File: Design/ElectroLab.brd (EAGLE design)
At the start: 175 x 100 mm, 229 parts, among them IC11 PAM8403, IC13 74HC08DD, IC14 74HC04DD, IC15 74HC32S14-13, IC3 LM324DTD, IC4 LM324DTD, IC6 MC74HC112ADR2G, IC7 MC74HC112ADR2G, IC8 TLC555CDR, IC9 TP4056, P1 SLIDE_POT_20MM, T1 MMBT2222A, T2 T_NPNMMBT2222A-1P_CHANGJ_SOT2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, T3 T_NPNMMBT2222A-1P_CHANGJ_SOT2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, T4 T_PNPMMBT5401_CHANGJ_SOT23-BEC, T5 T_PNPMMBT5401_CHANGJ_SOT23-BEC, U1 ADXL335, U2 GAS_SENSOR, U3 AMS1117-3.3VSMD, X8 USB-C-POWER

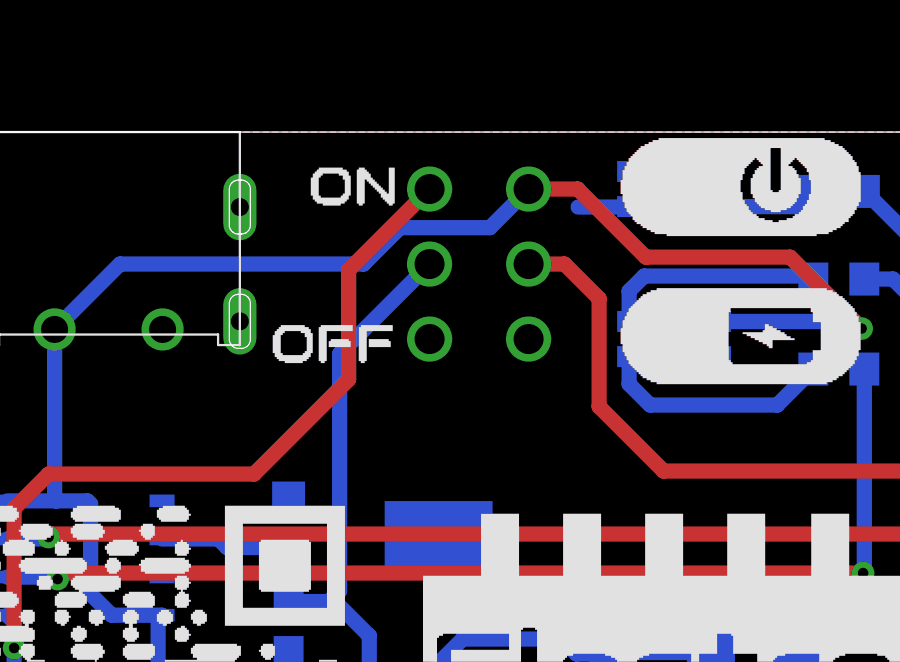
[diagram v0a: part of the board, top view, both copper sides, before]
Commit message: Added design files
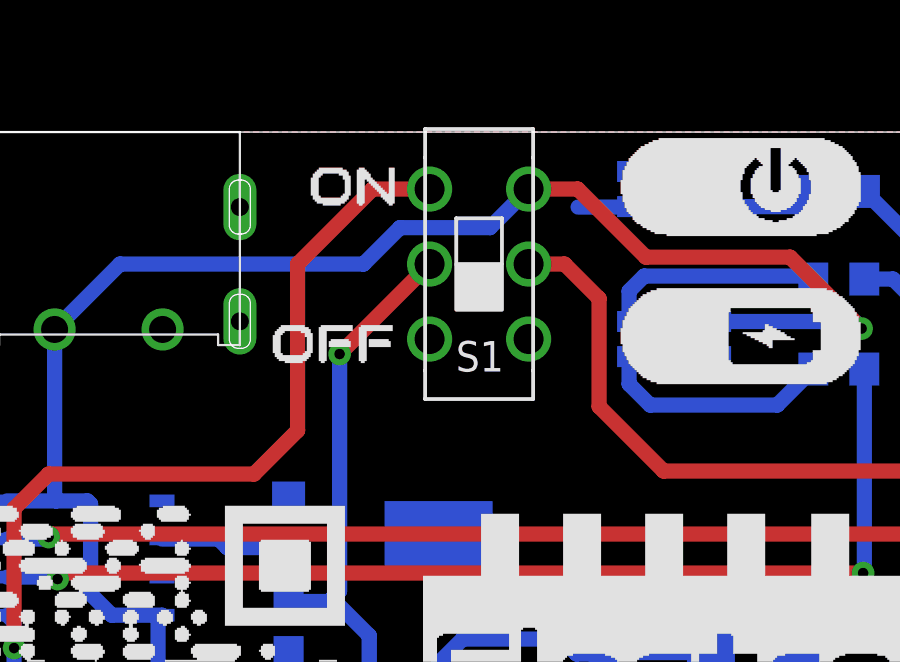
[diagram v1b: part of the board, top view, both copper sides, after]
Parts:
- S1: value (none) -> DPDT_JS202011CQN; device bt_electromech:DPDT_JS202011CQN -> SpaceDIY_electromechanical:DPDT_JS202011CQN
- flipped S1 to the top, turned to 90 degrees
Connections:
- net VBAT: now also S1.6; no longer S1.4
- net V_USB: now also S1.3; no longer S1.1
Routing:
- net VBAT: track 40.0 -> 41.1 mm
- net N$109: vias 0 -> 1
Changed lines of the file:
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@@
 <attribute name="VALUE" x="16.416" y="10.725" size="1.016" layer="28" rot="MR0" align="center"/>
 </element>
-<element name="S1" library="bt_electromech" package="DPDT_JS202011CQN" value="" x="28.85" y="95.6" smashed="yes" rot="MR270">
-<attribute name="NAME" x="28.9262" y="92.6738" size="1.016" layer="26" rot="MR270" align="center"/>
-<attribute name="VALUE" x="26.056" y="99.283" size="1.27" layer="28" rot="MR270"/>
+<element name="S1" library="SpaceDIY_electromechanical" package="DPDT_JS202011CQN" value="DPDT_JS202011CQN" x="28.85" y="95.6" smashed="yes" rot="R90">
+<attribute name="LCSC" value="C189615" x="28.85" y="95.6" size="1.778" layer="27" rot="R90" display="off"/>
+<attribute name="NAME" x="28.8738" y="92.5262" size="1.016" layer="25" rot="R180" align="center"/>
+<attribute name="VALUE" x="26.056" y="91.917" size="1.27" layer="27" rot="R90"/>
 </element>
 <element name="R31" library="SpaceDIY_passive_components" package="0603" value="470" x="40.85" y="98.02" smashed="yes" rot="MR0">
@@
 <contactref element="IC9" pad="5"/>
 <contactref element="C28" pad="1"/>
-<contactref element="S1" pad="4"/>
 <contactref element="J1" pad="1"/>
 <wire x1="13.35" y1="81.5" x2="13.35" y2="82.8" width="0.508" layer="16"/>
@@
 <wire x1="13.35" y1="87.45" x2="13.35" y2="82.8" width="0.508" layer="1"/>
 <via x="13.35" y="82.8" extent="1-16" drill="0.35"/>
-<wire x1="21.35" y1="88.6" x2="24.5" y2="91.75" width="0.508" layer="1"/>
-<wire x1="24.5" y1="95.4" x2="27.2" y2="98.1" width="0.508" layer="1"/>
-<wire x1="24.5" y1="91.75" x2="24.5" y2="95.4" width="0.508" layer="1"/>
+<wire x1="21.35" y1="88.6" x2="22.8" y2="90.05" width="0.508" layer="1"/>
+<wire x1="22.8" y1="90.05" x2="22.8" y2="95.6" width="0.508" layer="1"/>
+<contactref element="S1" pad="6"/>
+<wire x1="22.8" y1="95.6" x2="25.3" y2="98.1" width="0.508" layer="1"/>
+<wire x1="25.3" y1="98.1" x2="27.2" y2="98.1" width="0.508" layer="1"/>
 </signal>
 <signal name="N$104">
@@
 <wire x1="82.5" y1="45.2" x2="82.6" y2="45.1" width="0.508" layer="16"/>
 <contactref element="S1" pad="2"/>
-<wire x1="30.501" y1="95.6" x2="31.7" y2="95.6" width="0.508" layer="1"/>
 <wire x1="32.85" y1="94.45" x2="31.7" y2="95.6" width="0.508" layer="1"/>
 <via x="47.2" y="88.7" extent="1-16" drill="0.35"/>
@@
 <wire x1="47.2" y1="45" x2="47.2" y2="88.7" width="0.508" layer="16"/>
 <wire x1="35" y1="88.7" x2="32.85" y2="90.85" width="0.508" layer="1"/>
+<wire x1="31.7" y1="95.6" x2="30.501" y2="95.6" width="0.508" layer="1"/>
 </signal>
 <signal name="VOUT">
@@
 <wire x1="25.1886" y1="80.4012" x2="25.1886" y2="83.2114" width="0.508" layer="16"/>
 <wire x1="25.1886" y1="83.2114" x2="23.95" y2="84.45" width="0.508" layer="16"/>
-<wire x1="24.2" y1="92.601" x2="27.199" y2="95.6" width="0.508" layer="16"/>
+<wire x1="24.2" y1="92.601" x2="27.199" y2="95.6" width="0.508" layer="1"/>
 <wire x1="24.2" y1="84.7" x2="24.2" y2="92.601" width="0.508" layer="16"/>
+<via x="24.2" y="92.601" extent="1-16" drill="0.35"/>
 </signal>
 <signal name="N$102">
@@
 <contactref element="LED1" pad="3"/>
 <contactref element="LED1" pad="2"/>
-<contactref element="S1" pad="1"/>
 <wire x1="18.15" y1="81.5" x2="18.15" y2="83.765" width="0.508" layer="16"/>
 <wire x1="18.15" y1="83.765" x2="18.28" y2="83.895" width="0.508" layer="16"/>
@@
 <wire x1="14.7" y1="93.42" x2="14.7" y2="87.755" width="0.508" layer="16"/>
 <wire x1="14.7" y1="87.755" x2="14.75" y2="87.705" width="0.508" layer="16"/>
-<wire x1="30.5" y1="98.1" x2="32.13973125" y2="98.1" width="0.508" layer="1"/>
-<wire x1="32.13973125" y1="98.1" x2="34.40973125" y2="95.83" width="0.508" layer="1"/>
+<wire x1="34.40973125" y1="95.83" x2="32.13973125" y2="98.1" width="0.508" layer="1"/>
 <wire x1="14.7" y1="93.42" x2="16.88" y2="95.6" width="0.508" layer="16"/>
-<wire x1="29.213" y1="96.813" x2="30.5" y2="98.1" width="0.508" layer="16"/>
 <wire x1="26.213" y1="96.813" x2="29.213" y2="96.813" width="0.508" layer="16"/>
 <wire x1="16.88" y1="95.6" x2="25" y2="95.6" width="0.508" layer="16"/>
@@
 <wire x1="39.22" y1="95.83" x2="41.6" y2="93.45" width="0.508" layer="1"/>
 <wire x1="34.40973125" y1="95.83" x2="39.22" y2="95.83" width="0.508" layer="1"/>
+<contactref element="S1" pad="3"/>
+<wire x1="29.213" y1="96.813" x2="30.5" y2="98.1" width="0.508" layer="16"/>
+<wire x1="32.13973125" y1="98.1" x2="30.5" y2="98.1" width="0.508" layer="1"/>
 </signal>
 </signals>
